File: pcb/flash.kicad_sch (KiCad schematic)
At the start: 7 parts, among them U4 W25Q128JVS

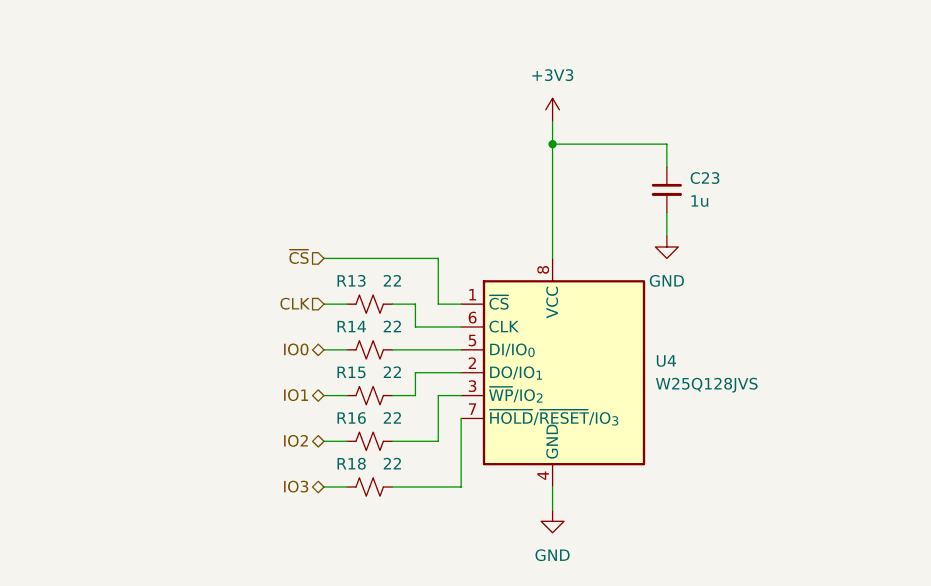
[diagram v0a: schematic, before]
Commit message: Update project
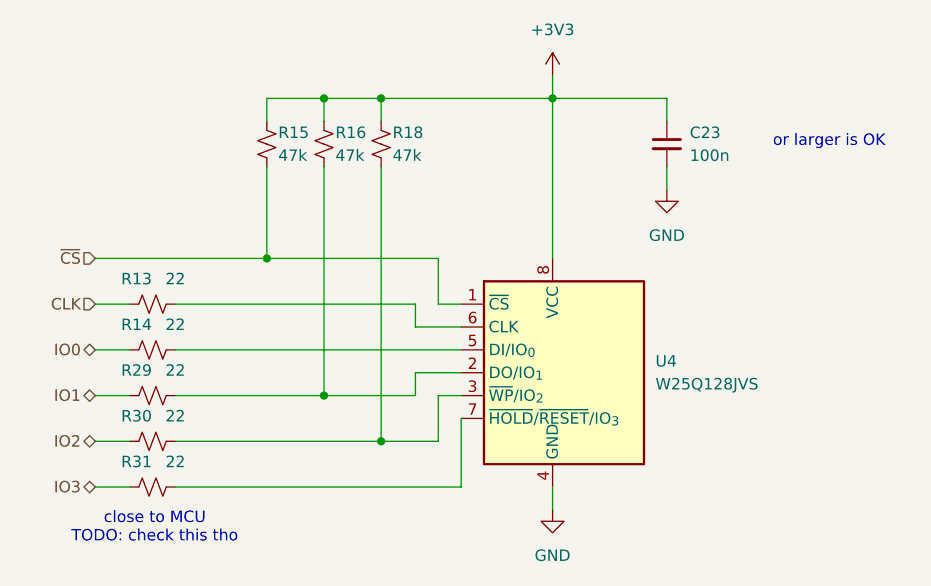
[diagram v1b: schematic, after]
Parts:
- added R29, R30, R31: 22, symbol Device:R_Small_US
- C23: value 1u -> 100n
- R15, R16, R18: value 22 -> 47k
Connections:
- net +3V3: now also R15.1, R16.1, R18.1
- net IO1: now also R29.1; no longer R15.1
- net IO2: now also R30.1; no longer R16.1
- net IO3: now also R31.1; no longer R18.1
- net ~{CS}: now also R15.2
- net at U4.2 (DO/IO_{1}): now also R16.2, R29.2; no longer R15.2
- net at R18.2: now also U4.3 (~{WP}/IO_{2}), R30.2; no longer U4.7 (~{HOLD}/~{RESET}/IO_{3})
- new net: R31.2, U4.7 (~{HOLD}/~{RESET}/IO_{3})
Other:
- note added: "close to MCU TODO: check this tho"
- note added: "or larger is OK"
- moved on the sheet: C23
